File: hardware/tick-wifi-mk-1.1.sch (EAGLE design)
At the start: 25 parts, among them IC1 MAX7219, IC2 MAX7219, IC3 74HC125, IC4 LD1117 5V, U1 Adafruit Feather HUZZAH ESP82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

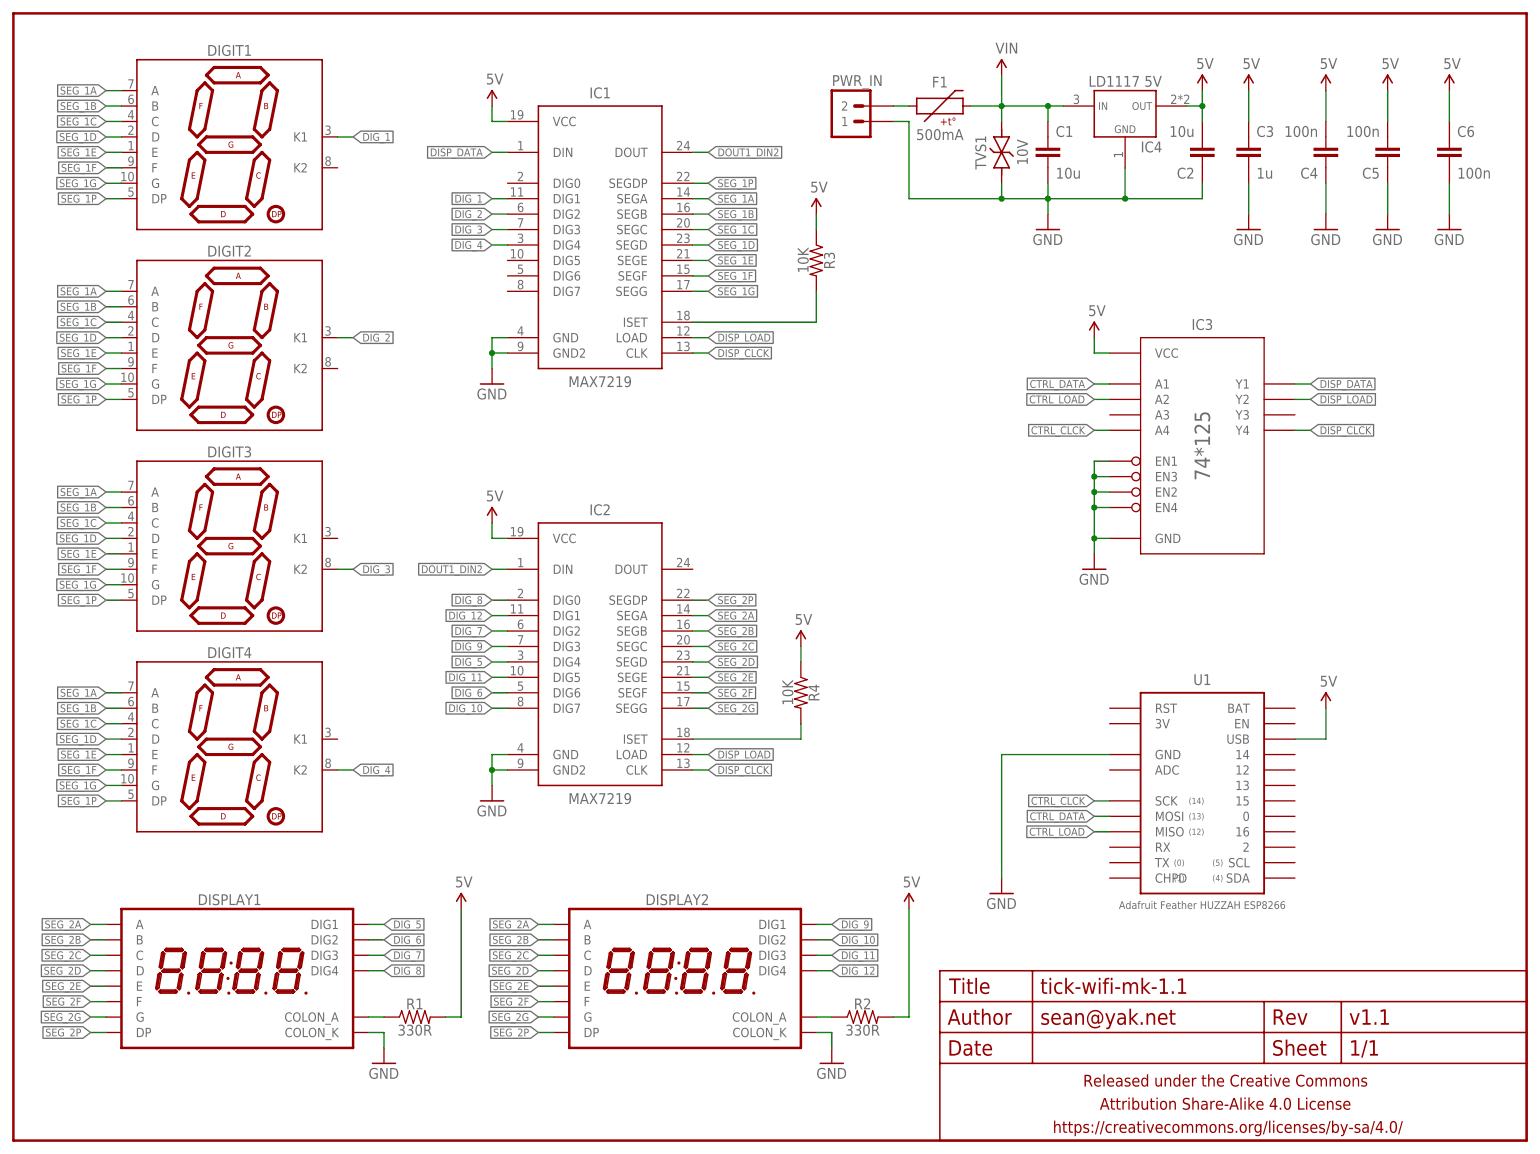
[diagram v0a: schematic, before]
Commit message: more wip
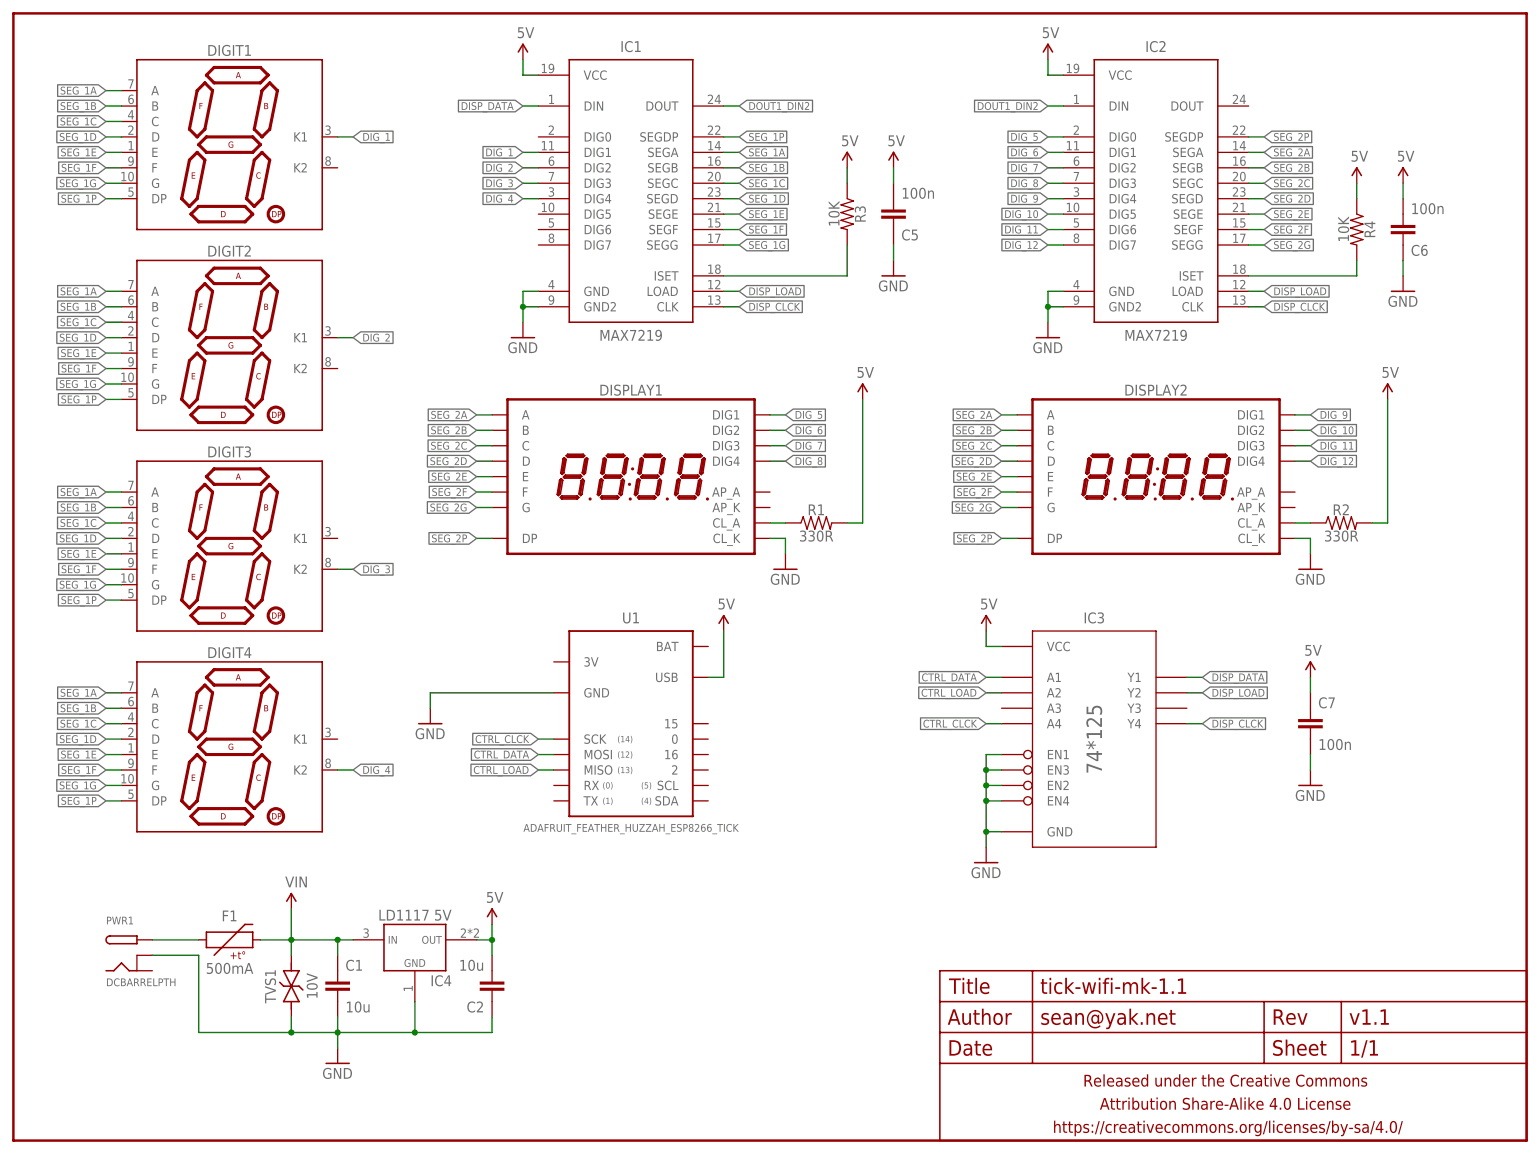
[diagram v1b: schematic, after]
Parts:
- removed C3: 1u, a_parts:CAPACITOR-CERAMICC0805
- removed C4: 100n, a_parts:CAPACITOR-CERAMICC0603
- removed PWR_IN: M02PTH-CENTERED-R+, A_butts:M02PTH-CENTERED-R+
- added C7: 100n, a_parts:CAPACITOR-CERAMICC0603
- added PWR1: DCBARRELPTH, a_parts:DCBARRELPTH
- DIGIT1, DIGIT2, DIGIT3, DIGIT4: device A_butts:7SEG_1DIGPTH-25.4MM-BARE -> a_parts:7SEG_1DIGPTH-25.4MM-BARE
- DISPLAY1, DISPLAY2: value 7SEG_4DIGIT_COLON14.2MM-CC -> 7SEG_4DIGIT_COLON_APOS; device a_parts:7SEG_4DIGIT_COLON14.2MM-CC -> a_parts:7SEG_4DIGIT_COLON_APOS
- F1: device A_butts:PTCPTC-1210 -> a_parts:PTCPTC-1210
- FRAME1: device A_butts:FRAME-LETTERNO_PACKAGE -> a_parts:FRAME-LETTERNO_PACKAGE
- TVS1: device A_butts:TVSSMA -> a_parts:TVSSMA
- U1: value Adafruit Feather HUZZAH ESP8266 -> ADAFRUIT_FEATHER_HUZZAH_ESP8266_TICK; device a_parts:ADAFRUIT_FEATHER_HUZZAH_ESP8266 -> a_parts:ADAFRUIT_FEATHER_HUZZAH_ESP8266_TICK
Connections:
- net 5V: now also C6.2, C7.1; no longer C3.1, C4.2, C6.1
- net DIG_10: now also IC2.DIG5; no longer IC2.DIG7
- net DIG_11: now also IC2.DIG6; no longer IC2.DIG5
- net DIG_12: now also IC2.DIG7; no longer IC2.DIG1
- net DIG_5: now also IC2.DIG0; no longer IC2.DIG4
- net DIG_6: now also IC2.DIG1; no longer IC2.DIG6
- net DIG_8: now also IC2.DIG3; no longer IC2.DIG0
- net DIG_9: now also IC2.DIG4; no longer IC2.DIG3
- net GND: now also C6.1, C7.2, DISPLAY1.CL_K, DISPLAY2.CL_K, PWR1.BRK; no longer C3.2, C4.1, C6.2, DISPLAY1.COLON_K, DISPLAY2.COLON_K, PWR_IN.1
- net N$1: now also PWR1.PWR; no longer PWR_IN.2
- net N$3: now also DISPLAY1.CL_A; no longer DISPLAY1.COLON_A
- net N$5: now also DISPLAY2.CL_A; no longer DISPLAY2.COLON_A
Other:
- moved on the sheet: C1, C2, C5, C6, F1, IC1, IC2, IC3, IC4, R1, R2, R3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
